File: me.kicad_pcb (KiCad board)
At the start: 2 copper layers, 8 parts, among them SW1 SW_Push, SW2 SW_Push, SW3 SW_Push, SW4 SW_Push, SW5 SW_Push, U1 XIAO-RP2040-DIP

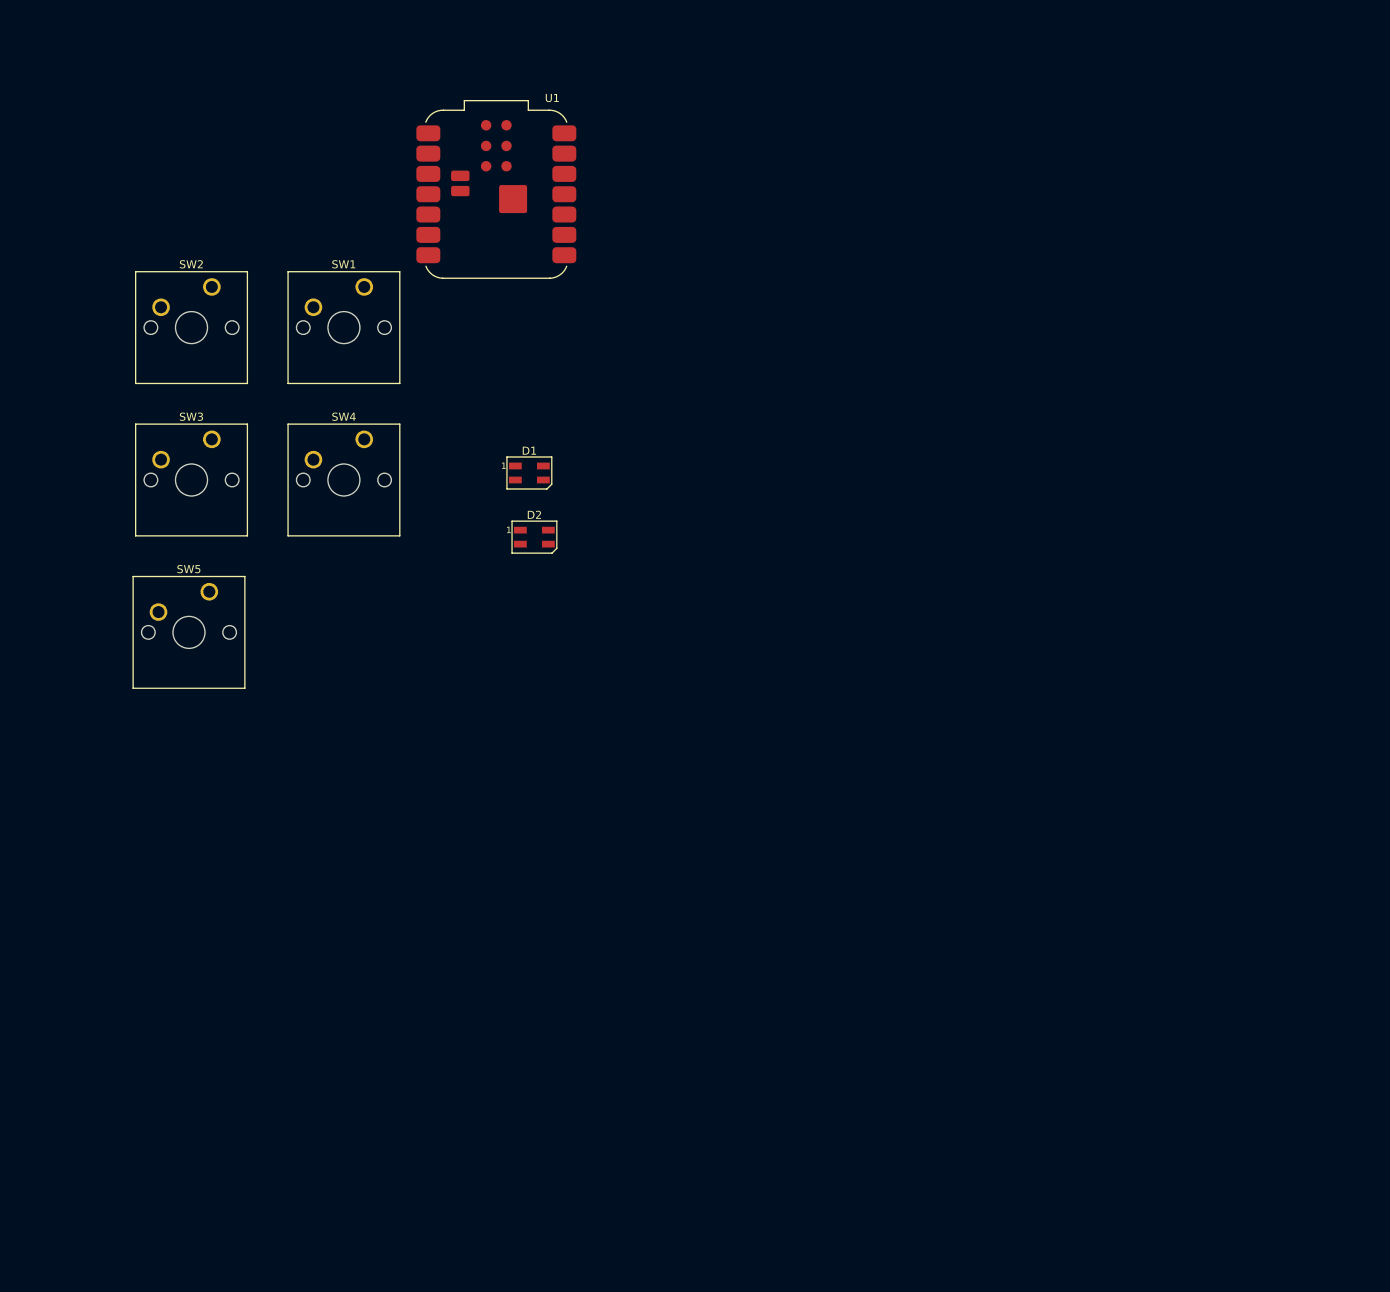
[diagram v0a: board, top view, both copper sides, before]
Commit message: erwovnojerwnhvonwejvew
wrjgvwjngvloekr3w
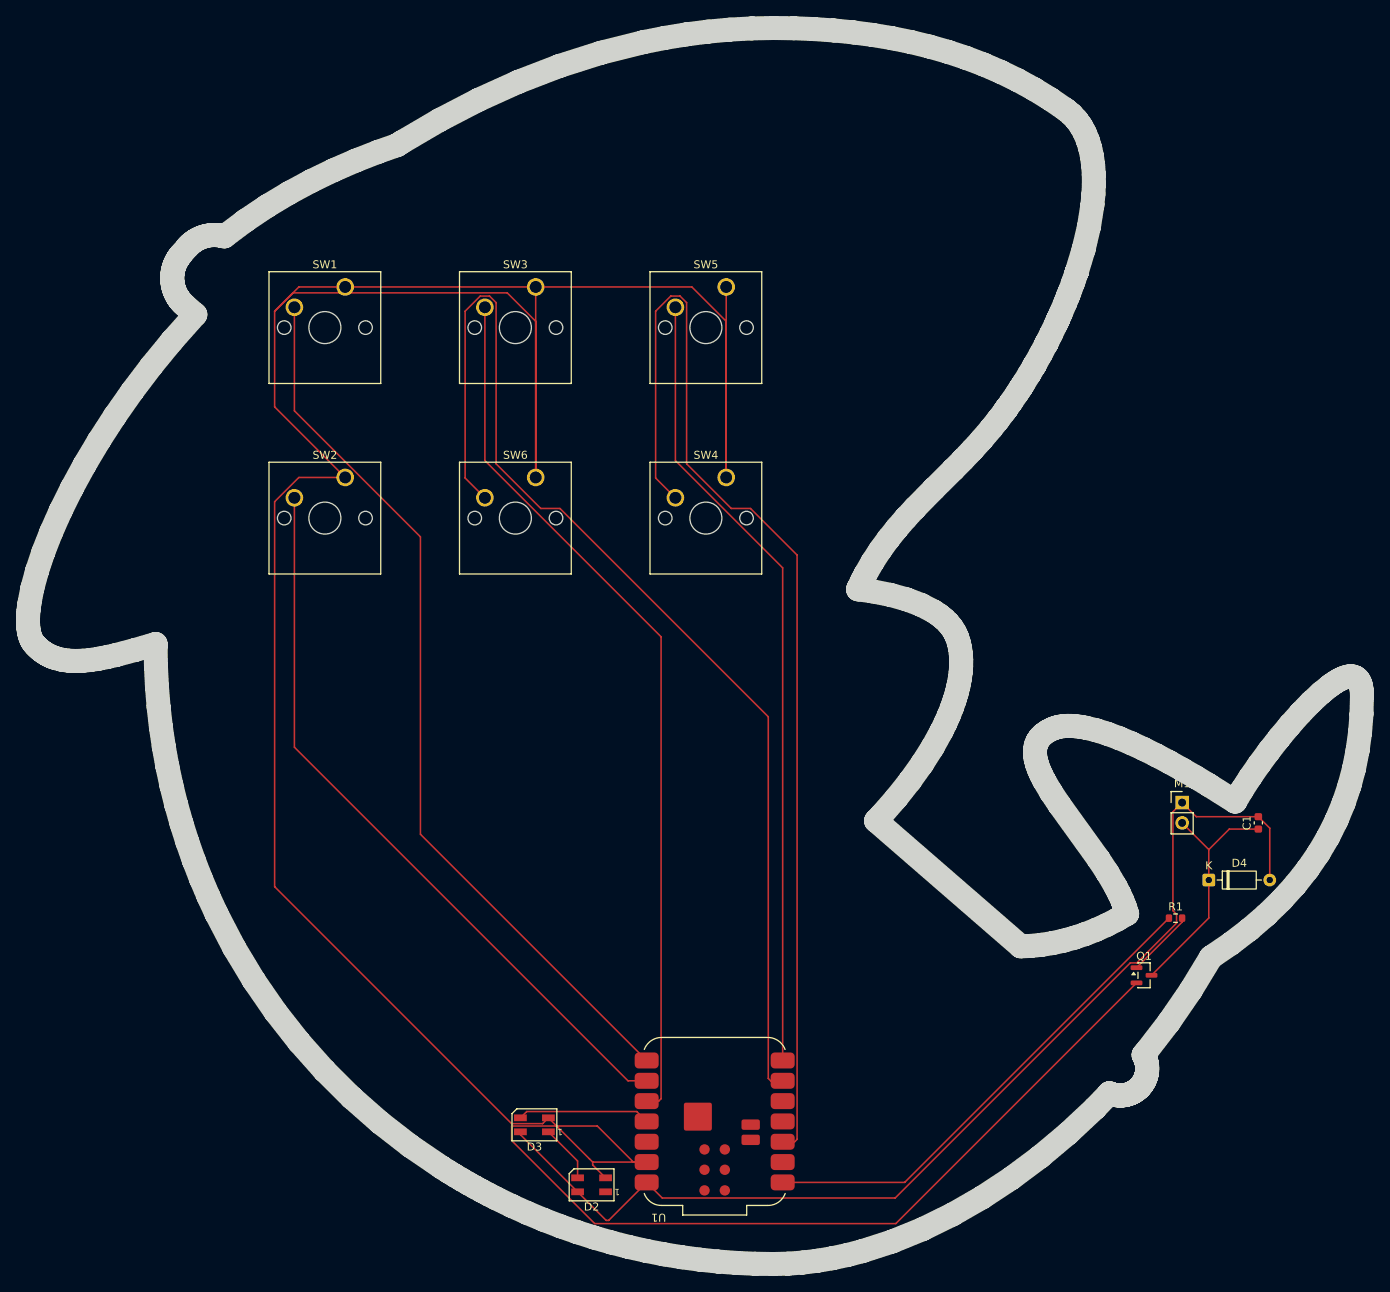
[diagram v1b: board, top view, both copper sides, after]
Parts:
- removed D1: SK6812MINI, LED_SMD:LED_SK6812MINI_PLCC4_3.5x3.5mm_P1.75mm
- added C1: 100 nF, Capacitor_SMD:C_0603_1608Metric, F.Cu at (231.0, 131.0)
- added D3: SK6812MINI, LED_SMD:LED_SK6812MINI_PLCC4_3.5x3.5mm_P1.75mm, F.Cu at (140.5, 168.7)
- added D4: 1N4148, Diode_THT:D_DO-35_SOD27_P7.62mm_Horizontal, F.Cu at (224.8, 138.1)
- added M1: Motor_DC, Connector_PinHeader_2.54mm:PinHeader_1x02_P2.54mm_Vertical, F.Cu at (221.5, 128.4)
- added Q1: AO3400A, Package_TO_SOT_SMD:SOT-23, F.Cu at (216.7, 150.0)
- added R1: 100 ohm, Resistor_SMD:R_0603_1608Metric, F.Cu at (220.6, 142.9)
- added SW6: SW_Push, Button_Switch_Keyboard:SW_Cherry_MX_1.00u_PCB, F.Cu at (140.7, 87.8)
- moved U1 119.1 mm to (163.0, 168.3), turned to 180 degrees
- moved D2 81.3 mm to (147.6, 176.2), turned to 180 degrees
- moved SW5 75.0 mm to (164.5, 64.0)
- moved SW4 45.5 mm to (164.5, 87.8)
- moved SW3 44.7 mm to (140.7, 64.0)
- moved SW2 29.1 mm to (116.8, 87.8)
- moved SW1 2.38 mm to (116.8, 64.0)
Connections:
- SW4 pad 2: Net-(U1-GPIO3/MOSI) -> Net-(U1-GPIO28/ADC2/A2)
- U1 pad 1: unconnected-(U1-GPIO26/ADC0/A0-Pad1) -> Net-(U1-GPIO26/ADC0/A0)
- U1 pad 11: Net-(U1-GPIO3/MOSI) -> Net-(D3-DIN)
- U1 pad 3: unconnected-(U1-GPIO28/ADC2/A2-Pad3) -> Net-(U1-GPIO28/ADC2/A2)
- U1 pad 5: Net-(D1-DIN) -> unconnected-(U1-GPIO6/SDA-Pad5)
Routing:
- net GND: track 0.00 -> 443.3 mm
- net Net-(U1-GPIO7/SCL): track 0.00 -> 143.7 mm
- net Net-(U1-GPIO28/ADC2/A2): track 0.00 -> 143.0 mm
- net +5V: track 0.00 -> 138.3 mm
- net Net-(U1-GPIO1/RX): track 0.00 -> 112.4 mm
- net Net-(U1-GPIO4/MISO): track 0.00 -> 110.0 mm
- net Net-(U1-GPIO0/TX): track 0.00 -> 99.7 mm
- net Net-(U1-GPIO2/SCK): track 0.00 -> 92.5 mm
- net Net-(U1-GPIO26/ADC0/A0): track 0.00 -> 62.0 mm
- net Net-(D4-K): track 0.00 -> 30.6 mm
- net Net-(D3-DIN): track 0.00 -> 16.6 mm
- net Net-(Q1-G): track 0.00 -> 8.55 mm
- net Net-(D2-DIN): track 0.00 -> 7.26 mm
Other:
- board outline added: 166.7 x 154.5 mm
